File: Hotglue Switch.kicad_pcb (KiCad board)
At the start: 2 copper layers, 26 x 10.2 mm, 10 parts, among them J3 BATTERY, J8 +OUTPUT, J9 -OUTPUT, M1 Screw, M2 Screw

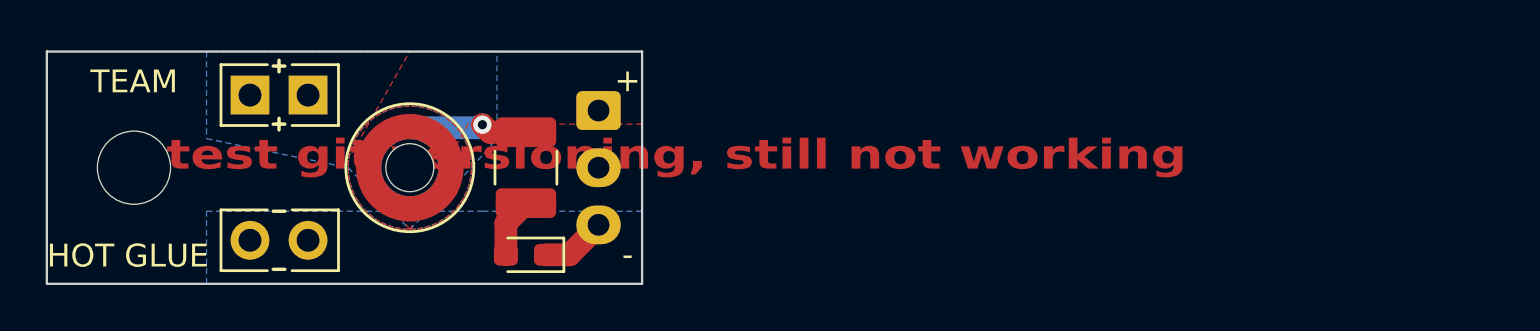
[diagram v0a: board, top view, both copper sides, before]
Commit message: commit of all modified files for rev 1.1, including gerbers, 3d step models, PCB, schematic, and project files.
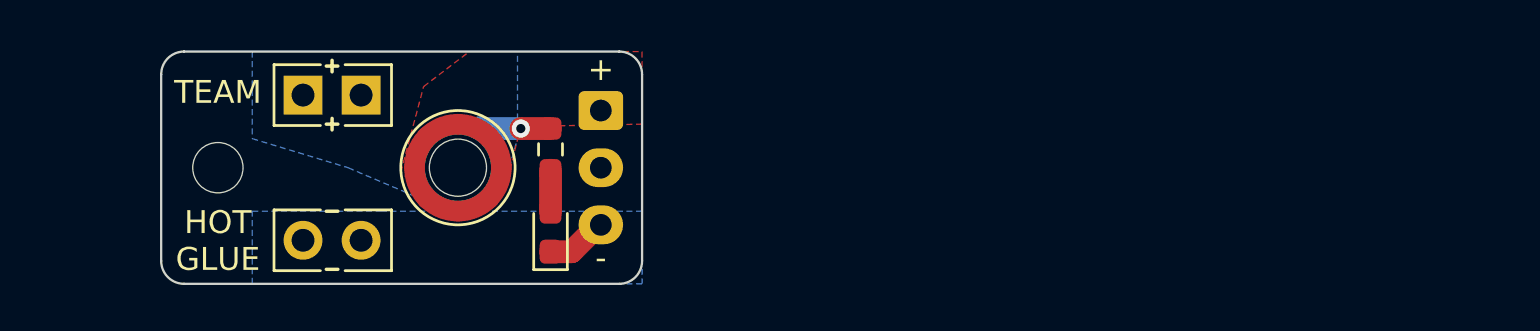
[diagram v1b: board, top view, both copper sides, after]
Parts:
- D1: value 150060GS75003 -> XL-1608UBC-06A
- H1: value MountingHole -> M2 MountingHole; footprint MountingHole:MountingHole_3.2mm_M3_DIN965 -> MountingHole:MountingHole_2.2mm_M2_DIN965
- H2: footprint Trent_Components_Library:screw_contact_3 -> Trent-footprints:Sinhoo-M1.6-screw-contact
- H4: value 9774010633R -> SMTSO1610MTJ; footprint Mounting_Wuerth:Mounting_Wuerth_WA-SMSI-M1.6_H1mm_9774010633 -> Trent-footprints:Mounting_Sinhoo_SMTSO1610MJT
- J3: footprint Trent_Components_Library:JST_XH_S3B-XH-A-1_1x03_P2.50mm_Horizontal_Aliexpress -> Trent-footprints:JST_XH_S3B-XH-A-1_1x03_P2.50mm_Horizontal_Aliexpress
- J8: footprint Trent_Components_Library:PinHeader_1x02_P2.54mm_Vertical Positive -> Trent-footprints:PinHeader_1x02_P2.54mm_Vertical Positive
- J9: footprint Trent_Components_Library:PinHeader_1x02_P2.54mm_Vertical Negative -> Trent-footprints:PinHeader_1x02_P2.54mm_Vertical Negative
- M1: value Screw -> M1.6 Screw; footprint Trent_Components_Library:Screw M1.6 -> Trent-footprints:Screw M1.6
- M2: value Screw -> M2 Screw; footprint Trent_Components_Library:Screw M3 -> Trent-footprints:Screw M2
- R1: value 560112140008 -> RC0603FR-07390RL; footprint Resistor_SMD:R_1210_3225Metric_Pad1.30x2.65mm_HandSolder -> Resistor_SMD:R_0603_1608Metric_Pad0.98x0.95mm_HandSolder
- moved H1 3.67 mm to (72.2, 50.8)
- moved M2 3.67 mm to (72.2, 50.8)
- moved J8 2.32 mm to (76.0, 47.6)
- moved J9 2.32 mm to (76.0, 54.0)
- moved H2 2.11 mm to (82.8, 50.8)
- moved H4 2.11 mm to (82.8, 50.8)
- moved M1 2.11 mm to (82.8, 50.8)
- moved D1 1.48 mm to (86.8, 53.6), turned to 90 degrees
- moved R1 1.34 mm to (86.8, 50.0)
- moved J3 0.10 mm to (89.0, 48.3)
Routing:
- net /BATT SWITCH: track 5.27 -> 3.13 mm
- net Net-(D1-A): track 2.62 -> 1.81 mm
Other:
- board size 26 x 10.2 mm -> 21 x 10.2 mm
- board text added: "ANT SWITCH"
- board text added: "v1.1"
- board text removed: "ANTSWITCH"
- board text removed: "test git versioning, still not working"
- board text removed: "v1.0"
